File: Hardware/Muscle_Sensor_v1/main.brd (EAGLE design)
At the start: 76 x 42 mm, 35 parts, among them IC1 TL084D, IC2 TL7660D, IC3 LM358D, U1 AD8221AR

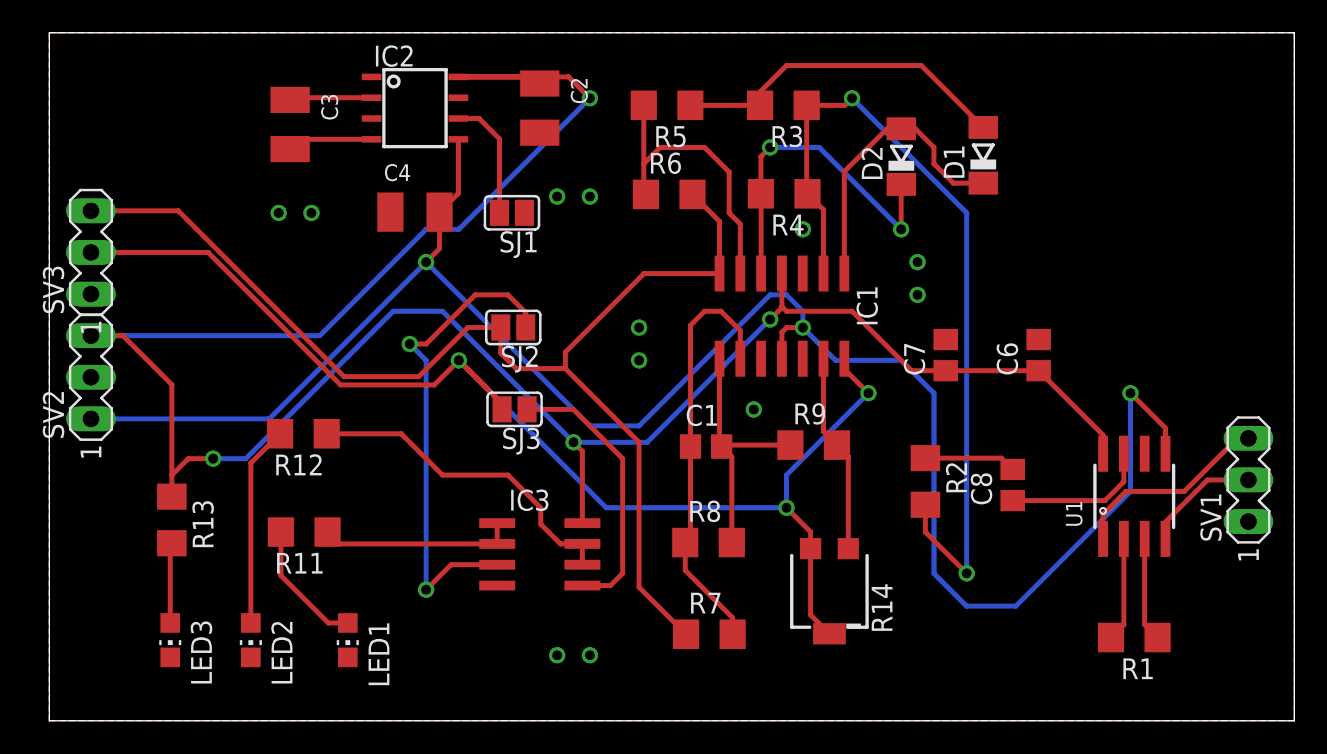
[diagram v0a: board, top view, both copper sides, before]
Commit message: Update Muscle_Sensor_v1
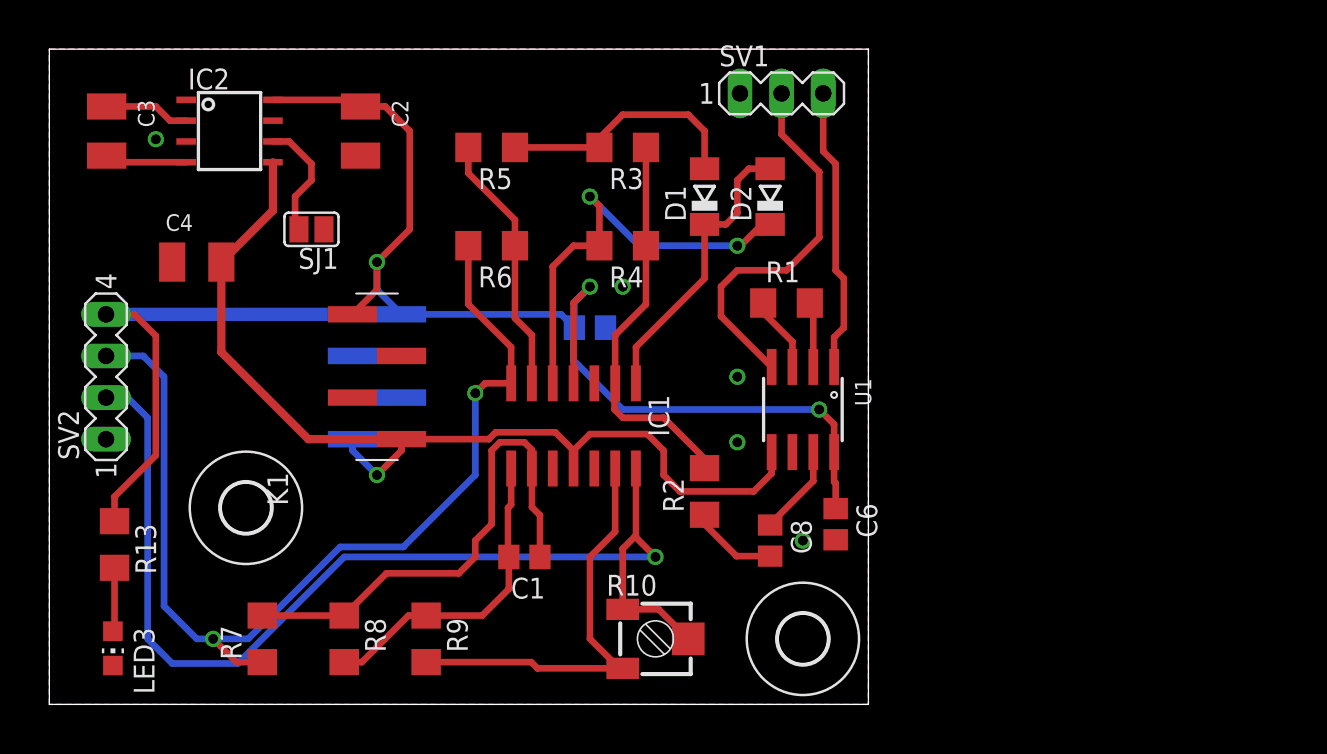
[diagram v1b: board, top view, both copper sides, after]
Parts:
- removed IC3: LM358D, linear:SO08
- removed LED1, LED2: (no value), led:CHIP-LED0805
- removed R11, R12: 330R, rcl:R1206
- removed R14: (no value), pot:SM-42/43B
- removed SJ2, SJ3: (no value), jumper:SJ
- removed SV3: (no value), con-lstb:MA03-1
- added H1, H2: MOUNT-HOLE3.0, holes:3,0
- added K1, K2: 61000418221, Wurth_Elektronik_Electromechanic_Board_to_Board_Connectors_rev15c:61000418221
- added R10: (no value), rcl:RTRIM3314J
- SV2: device con-lstb:MA03-1 -> con-lstb:MA04-1
- moved SV1 37.0 mm to (44.7, 38.3), turned to 0 degrees
- moved R1 29.5 mm to (45.0, 25.5), turned to 0 degrees
- moved R7 27.3 mm to (13.0, 5.00), turned to 90 degrees
- moved R9 26.5 mm to (23.0, 5.00), turned to 270 degrees
- moved R8 23.0 mm to (18.0, 5.00), turned to 270 degrees
- moved C7 21.8 mm to (33.0, 24.0), flipped to the bottom, turned to 180 degrees
- moved U1 20.9 mm to (46.0, 19.0), turned to 180 degrees
- moved D1 17.2 mm to (40.0, 32.0)
- moved C6 16.1 mm to (48.0, 12.0), turned to 270 degrees
- moved C8 15.2 mm to (44.0, 11.0), turned to 270 degrees
- moved IC1 14.4 mm to (32.0, 18.0)
- moved C4 13.7 mm to (9.00, 28.0)
- moved R2 13.5 mm to (40.0, 14.0), turned to 90 degrees
- moved C1 13.0 mm to (29.0, 10.0), turned to 180 degrees
- moved SJ1 12.3 mm to (16.0, 30.0)
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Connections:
- removed net N$12: IC3.3, SJ2.1
- removed net N$15: IC3.5, SJ3.1
- removed net N$16: IC3.6, IC3.7, R12.1
- removed net N$17: IC3.1, IC3.2, R11.1
- removed net N$18: LED1.A, R11.2
- removed net N$20: LED2.A, R12.2
- net GND: now also K1.2, K1.3, K2.2, K2.3, SV2.1; no longer IC3.4, LED1.C, LED2.C, SV2.2, SV3.1
- net N$11: now also R10.1; no longer R14.3
- net RECT: now also SV2.3; no longer SJ2.2, SV3.3
- net SIG: now also R10.2, R10.3, SV2.2; no longer R14.1, R14.2, SJ3.2, SV3.2
- net V+: now also K1.4, K2.4, SV2.4; no longer IC3.8, SV2.3
- net V-: now also K1.1, K2.1; no longer SV2.1
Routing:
- net V-: track 114.8 -> 60.6 mm, vias 3 -> 1
- net V+: track 142.5 -> 104.4 mm, vias 4 -> 3
- net N$12: track 30.1 -> 0.00 mm, vias 2 -> 0
- net N$1: track 50.8 -> 24.1 mm, vias 2 -> 0
- net N$16: track 20.2 -> 0.00 mm
- net N$15: track 16.9 -> 0.00 mm
- net MID: track 7.27 -> 23.2 mm
- net N$11: track 12.2 -> 25.9 mm
- net SIG: track 79.0 -> 66.3 mm, vias 3 -> 1
- net N$20: track 12.3 -> 0.00 mm
- net N$17: track 11.9 -> 0.00 mm
- net RECT: track 73.5 -> 62.5 mm, vias 0 -> 2
- net N$18: track 7.94 -> 0.00 mm
- net N$7: track 20.8 -> 26.5 mm
- net N$6: track 20.9 -> 15.5 mm
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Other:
- board size 76 x 42 mm -> 50 x 40 mm
